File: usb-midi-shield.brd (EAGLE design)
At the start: 31 parts, among them IC1 ATMEGA32U2-TQFP, U1 ARDUINOR3NODIM

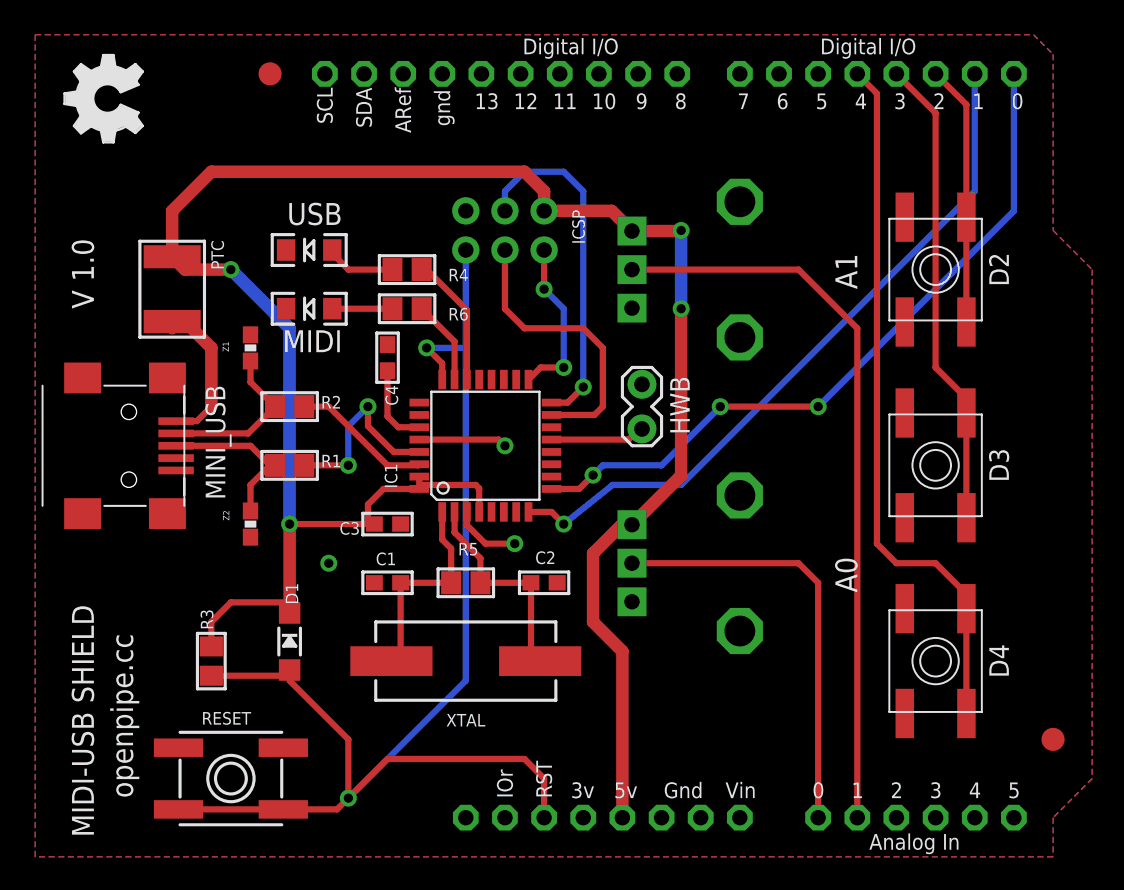
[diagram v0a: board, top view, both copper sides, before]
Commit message: changed to v1.1
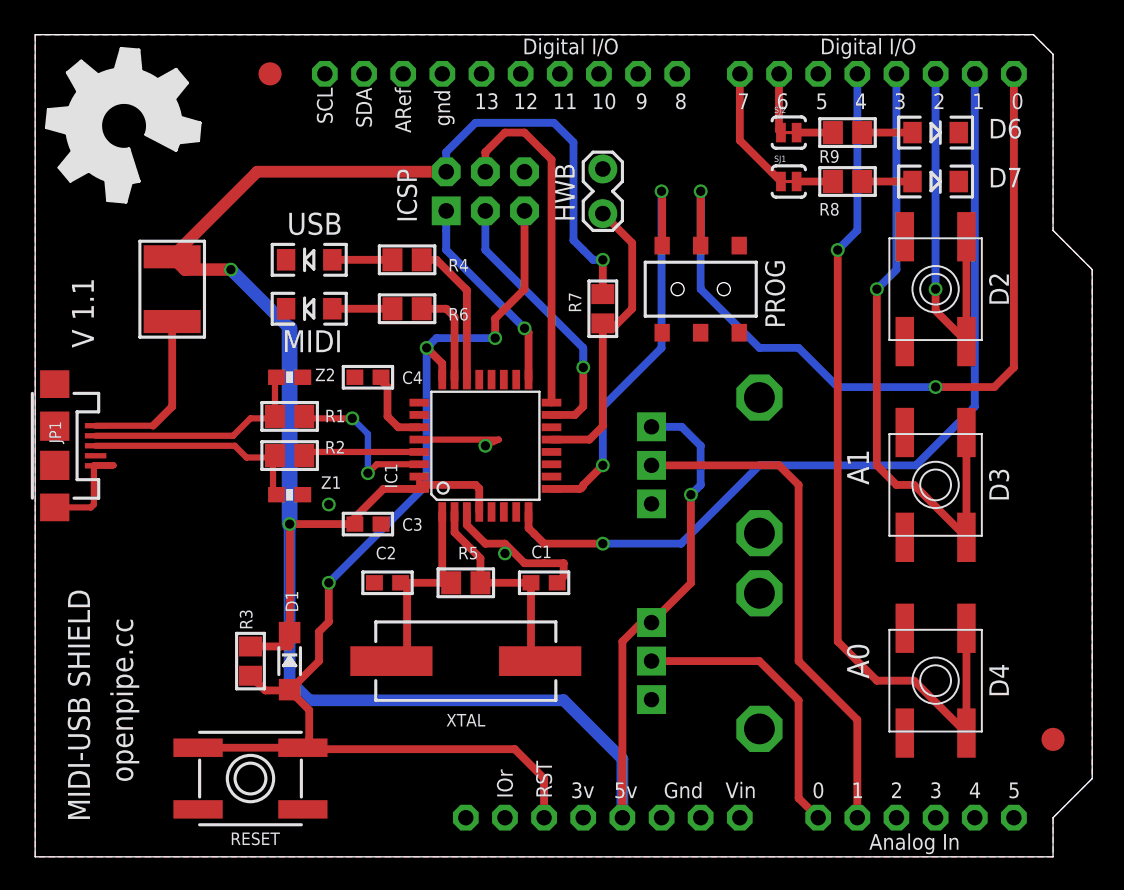
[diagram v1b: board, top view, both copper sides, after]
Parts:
- removed MINI_USB: (no value), adafruit:USB-MINIB
- added D6: GREEN, SparkFun-LED:LED-1206
- added D7: RED, SparkFun-LED:LED-1206
- added JP1: USB-MICROB, SparkFun-Connectors:USB-MICROB
- added PROG: AYZ0202AGRLC, SparkFun-Electromechanical:AYZ0202
- added R7: 10k, microbuilder:0805
- added R8, R9: 1k, microbuilder:0805
- added SJ1, SJ2: SOLDERJUMPERTRACE, SparkFun-Passives:SJ_2S-TRACE
- ICSP: value (none) -> AVR_SPI_PRG_6NS; device microbuilder:2X03_ROUND_70MIL -> SparkFun-Connectors:2X3-NS
- LOGO1: value OSHW_LOGO_FILLX0200-NT -> OSHW_LOGO_FILLX0350-NT; device ohw-logo:OSHW_FILLX200_NOTEXT -> ohw-logo:OSHW_FILLX350_NOTEXT
- moved A1 12.8 mm to (54.6, 30.5)
- moved HWB 11.7 mm to (44.5, 47.0), turned to 90 degrees
- moved C1 10.2 mm to (40.6, 22.9), turned to 180 degrees
- moved C2 10.2 mm to (30.5, 22.9), turned to 0 degrees
- moved Z1 9.86 mm to (24.1, 28.6), turned to 0 degrees
- moved Z2 9.86 mm to (24.1, 36.2), turned to 0 degrees
- moved A0 6.48 mm to (54.6, 17.8)
- moved LOGO1 5.68 mm to (12.1, 46.4), turned to 40 degrees
- moved R1 3.18 mm to (24.1, 33.7)
- moved R2 3.18 mm to (24.1, 31.1)
- moved ICSP 2.84 mm to (36.8, 48.3), turned to 0 degrees
- moved R3 2.54 mm to (21.6, 17.8)
- moved C4 1.80 mm to (29.2, 36.2), turned to 180 degrees
- moved D2 1.27 mm to (66.0, 41.9)
- moved C3 1.27 mm to (29.2, 26.7)
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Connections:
- net N$14 renamed MISO
- net N$17 renamed SCK
- net N$19 renamed MOSI
- net N$8 renamed ARDUINO_TX
- removed net N$24: HWB.2, IC1.13
- removed net N$25: C1.2, IC1.1, R5.1, XTAL.2
- removed net N$6: IC1.29, R1.2
- removed net N$7 (its old number): IC1.9, U1.D0
- new net ARDUINO_RX: IC1.9, PROG.1
- new net D-: IC1.29, R2.2
- new net N$1: HWB.1, IC1.13, R7.1
- new net N$23: JP1.D-, R1.1, Z2.1
- new net N$29: R8.2, SJ1.2
- new net N$30: D7.A, R8.1
- new net N$32: R9.2, SJ2.2
- new net N$33: D6.A, R9.1
- new net N$34: SJ2.1, U1.D6
- new net N$36: SJ1.1, U1.D7
- new net N$37: PROG.2, U1.D0
- net GND: now also C4.2, D6.C, D7.C, HWB.2, JP1.GND, JP1.MT1, JP1.MT2; no longer C4.1, HWB.1, MINI_USB.GND
- net N$10: now also JP1.VBUS; no longer MINI_USB.VBUS
- net N$2: now also C1.2; no longer C2.2
- net N$3: now also JP1.D+; no longer MINI_USB.D-
- net N$4: now also C2.2, IC1.1, R5.1, XTAL.2; no longer IC1.30, R2.2
- net N$5: now also IC1.30, R1.2; no longer MINI_USB.D+, R1.1, Z2.1
- net N$9: now also C4.1; no longer C4.2
- net VCC: now also R7.2
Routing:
- net N$37: track 0.00 -> 52.7 mm, vias 0 -> 2
- net N$7 (its old number): track 46.4 -> 0.00 mm, vias 3 -> 0
- net ARDUINO_RX: track 0.00 -> 26.9 mm, vias 0 -> 2
- net VCC: track 133.7 -> 158.3 mm
- net N$1: track 0.00 -> 19.4 mm
- net N$23: track 0.00 -> 14.7 mm
- net N$26: track 47.9 -> 33.2 mm
- net N$25: track 14.2 -> 0.00 mm
- net RESET: track 87.1 -> 75.9 mm, vias 2 -> 3
- net GND: track 10.2 -> 20.9 mm
- net ARDUINO_TX: track 45.7 -> 55.7 mm
- net N$6: track 12.5 -> 2.54 mm, vias 2 -> 0
- net N$8: track 30.7 -> 40.5 mm, vias 0 -> 1
- net N$27: track 27.8 -> 18.7 mm
- net N$20: track 45.9 -> 55.0 mm, vias 0 -> 1
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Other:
- board outline added: 68.6 x 53.3 mm
- board text added: "V 1.1"
- board text removed: "V 1.0"
